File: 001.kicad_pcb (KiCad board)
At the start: 2 copper layers, 162.6 x 57.2 mm, 35 parts, among them CN11 02-XH-A, CN12 02-XH-A, CN21 02-XH-A, CN22 02-XH-A, J11 RJ45, J12 RJ45, J21 RJ45, J22 RJ45, K11 JQC-3FF, K21 JQC-3FF, U11 TLP222A, U21 TLP222A

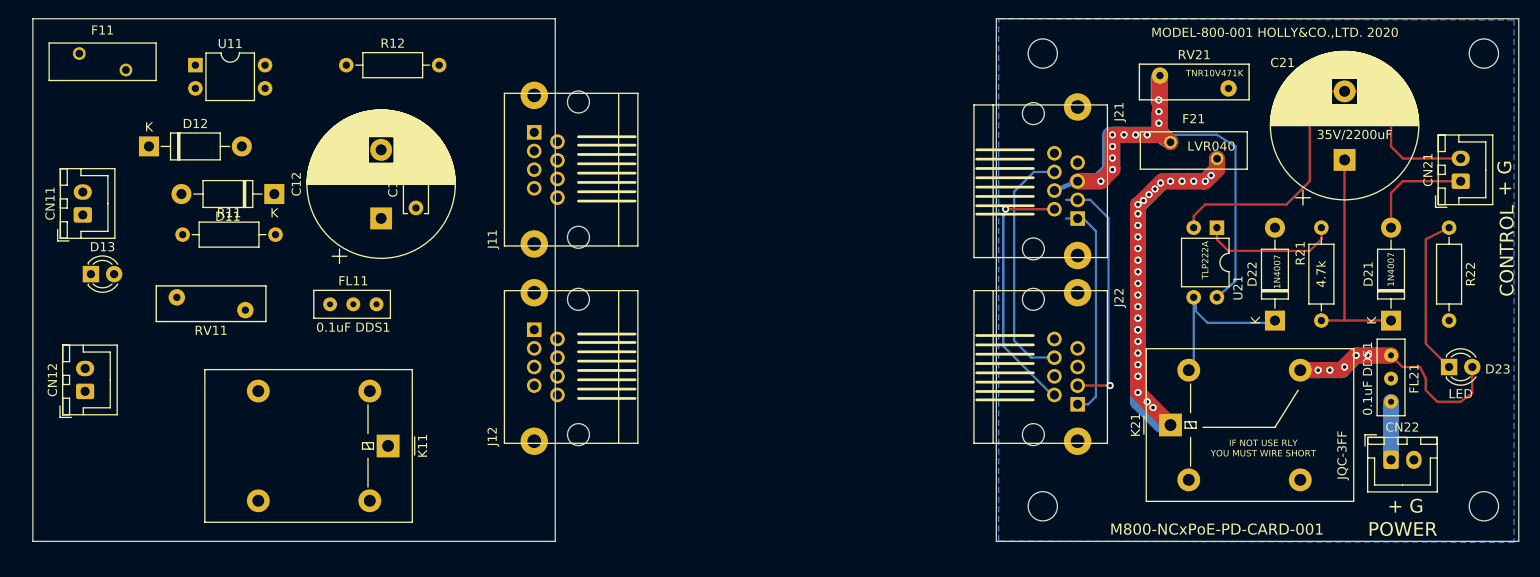
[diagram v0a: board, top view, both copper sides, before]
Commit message: 一応完成、これからガーバー
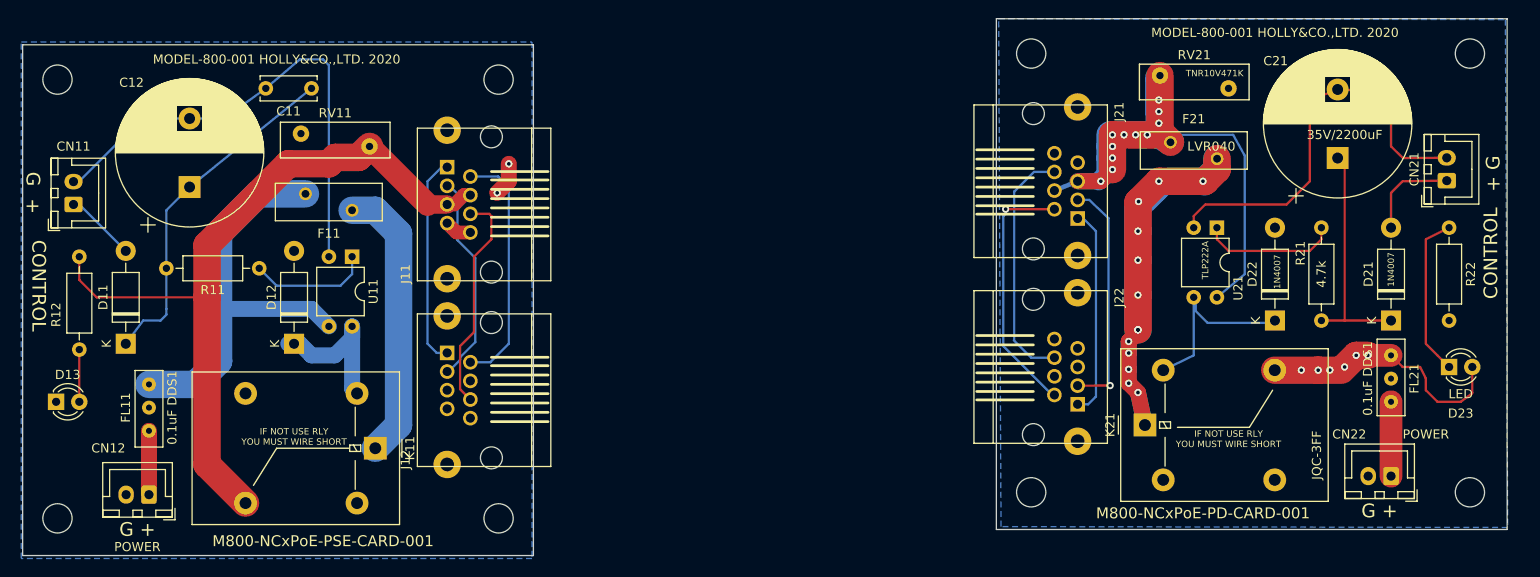
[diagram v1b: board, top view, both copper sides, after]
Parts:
- added REF**: MountingHole_3.2mm_M3, MountingHole:MountingHole_3.2mm_M3, F.Cu at (122.1, 111.8)
- added REF**: MountingHole_3.2mm_M3, MountingHole:MountingHole_3.2mm_M3, F.Cu at (73.8, 111.8)
- added REF**: MountingHole_3.2mm_M3, MountingHole:MountingHole_3.2mm_M3, F.Cu at (73.8, 63.8)
- added REF**: MountingHole_3.2mm_M3, MountingHole:MountingHole_3.2mm_M3, F.Cu at (122.1, 63.8)
- moved R12 35.9 mm to (76.2, 83.2), turned to 270 degrees
- moved F11 34.4 mm to (106.0, 78.1), turned to 180 degrees
- moved U11 27.1 mm to (106.0, 83.2), turned to 270 degrees
- moved D12 26.8 mm to (99.7, 92.7), turned to 90 degrees
- moved RV11 26.8 mm to (108.0, 71.1), turned to 180 degrees
- moved FL11 25.0 mm to (83.8, 99.7), turned to 90 degrees
- moved D11 23.1 mm to (81.3, 92.7), turned to 90 degrees
- moved C12 21.2 mm to (88.3, 75.6)
- moved C11 17.4 mm to (101.6, 64.8), turned to 180 degrees
- moved D13 14.5 mm to (73.7, 99.1)
- moved CN12 13.3 mm to (83.8, 109.2), turned to 180 degrees
- moved J11 10.3 mm to (121.3, 77.5)
- moved J12 9.86 mm to (121.3, 97.8)
- moved R11 9.16 mm to (95.9, 84.5), turned to 180 degrees
- moved K21 2.79 mm to (192.8, 101.6)
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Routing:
- net /PSE_PWR: track 0.00 -> 83.6 mm
- net Net-(C11-Pad2): track 0.00 -> 54.3 mm
- net Net-(F11-Pad2): track 0.00 -> 46.8 mm
- net Net-(C11-Pad1): track 0.00 -> 38.2 mm
- net Net-(F11-Pad1): track 0.00 -> 30.7 mm
- net /PSEBUS2: track 0.00 -> 26.9 mm
- net /PSEBUS4: track 0.00 -> 24.4 mm
- net /PSEBUS1: track 0.00 -> 23.1 mm
- net /PSEBUS3: track 0.00 -> 23.1 mm
- net Net-(D12-Pad1): track 0.00 -> 17.1 mm
- net Net-(R11-Pad1): track 0.00 -> 13.4 mm
- net Net-(CN22-Pad1): track 6.35 -> 16.3 mm
- net Net-(CN11-Pad1): track 0.00 -> 7.82 mm
- net Net-(CN12-Pad1): track 0.00 -> 6.98 mm
- net /PSE_GND: track 0.00 -> 6.66 mm, vias 0 -> 2
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- added copper zone on B.Cu, net /PSE_GND
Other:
- board size 162.6 x 57.2 mm -> 162.4 x 58.7 mm
- board text added: "G +"
- board text added: "M800-NCxPoE-PSE-CARD-001"
